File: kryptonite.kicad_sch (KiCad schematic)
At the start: 27 parts, among them J1 Conn_01x04_Pin, P1 USB_C_Plug_USB2.0, SW1 SW_Push, U1 STM32F072CBUx, U2 ATECC608B-MAHDA, U3 MCP1700x-330xxTT, U4 USBLC6-2SC6, Y1 8MHz

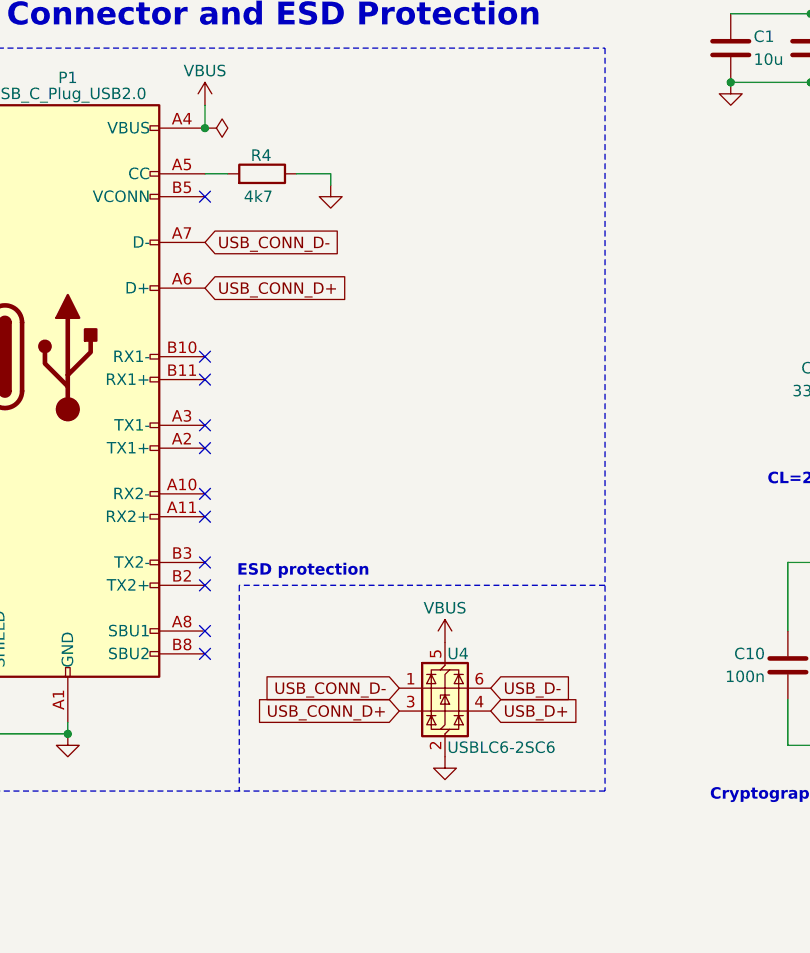
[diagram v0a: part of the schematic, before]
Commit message: Add files via upload
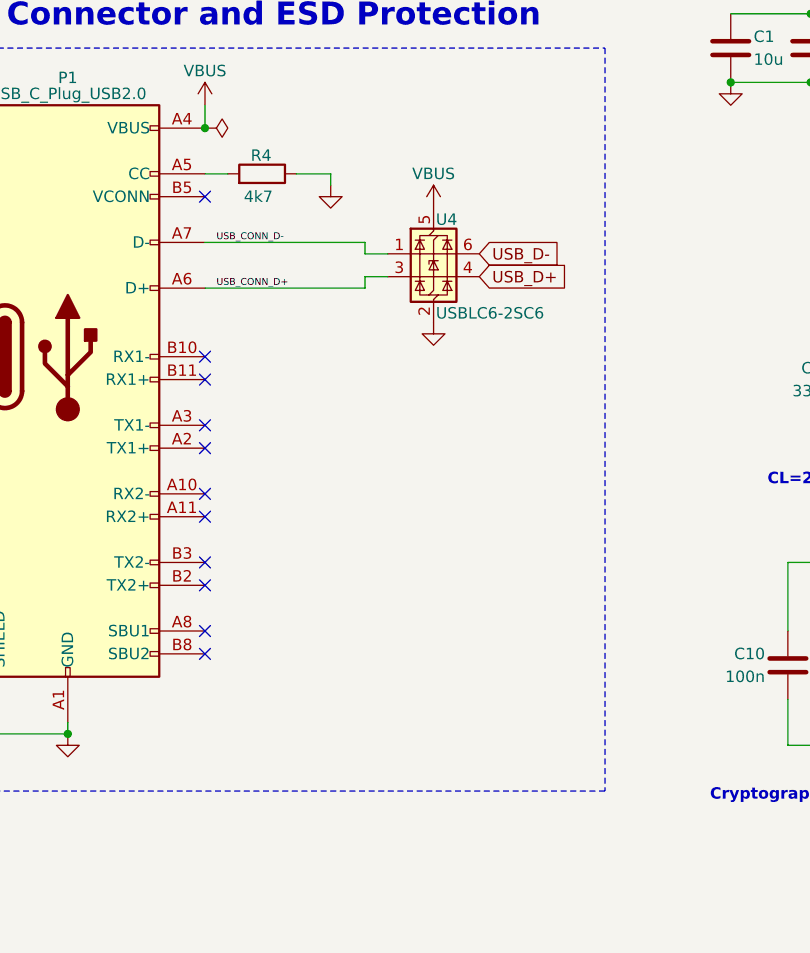
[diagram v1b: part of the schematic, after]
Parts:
- C1, C11, C12: Distributer Link (none) -> https://www.lcsc.com/product-detail/Multilayer-Ceramic-Capa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; LCSC (none) -> C466781; Manufacturer (none) -> SANYEAR; Manufacturer Part Number (none) -> C0603X5R106M160NT
- C10, C2, C3, C4, C5, C6, C7: Distributer Link (none) -> https://www.lcsc.com/product-detail/Multilayer-Ceramic-Capa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; LCSC (none) -> C6119799; Manufacturer (none) -> HRE; Manufacturer Part Number (none) -> CGA0402X7R104K160GT
- C8, C9: Distributer Link (none) -> https://www.lcsc.com/product-detail/Multilayer-Ceramic-Capa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; LCSC (none) -> C696910; Manufacturer (none) -> CCTC; Manufacturer Part Number (none) -> TCC0402COG330J500AT
- D1: LCSC (none) -> C965799
- J1: LCSC (none) -> C7430360
- P1: LCSC (none) -> C530605; Manufacturer Korean Hroparts Elec -> Korean Hroparts Elec
- R1, R5: LCSC (none) -> C60490
- R2, R3, R4: LCSC (none) -> C25940
- R6: LCSC (none) -> C2906961
- SW1: LCSC (none) -> C318884
- U1: LCSC (none) -> C92504
- U2: LCSC (none) -> C1518773
- U3: LCSC (none) -> C39051
- U4: LCSC (none) -> C7519
- Y1: LCSC (none) -> C720915
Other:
- note removed: "ESD protection"
- moved on the sheet: U4
